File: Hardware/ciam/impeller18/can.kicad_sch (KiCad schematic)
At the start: 66 parts, among them J24 PLS-5, J25 PLS-5, J5 430450400, J6 430450400, SW4 MSS-12D16, SW5 MSS-12D16, U11 ISO1050DUB, U12 ISO1050DUB, U13 MCP2515-I/SO, U14 B0505MT-1WR4, U15 ISO1050DUB, U16 ISO1050DUB, U17 MCP2515-I/SO, U18 B0505MT-1WR4, Y3 X322516MLB4SI, Y4 X322516MLB4SI

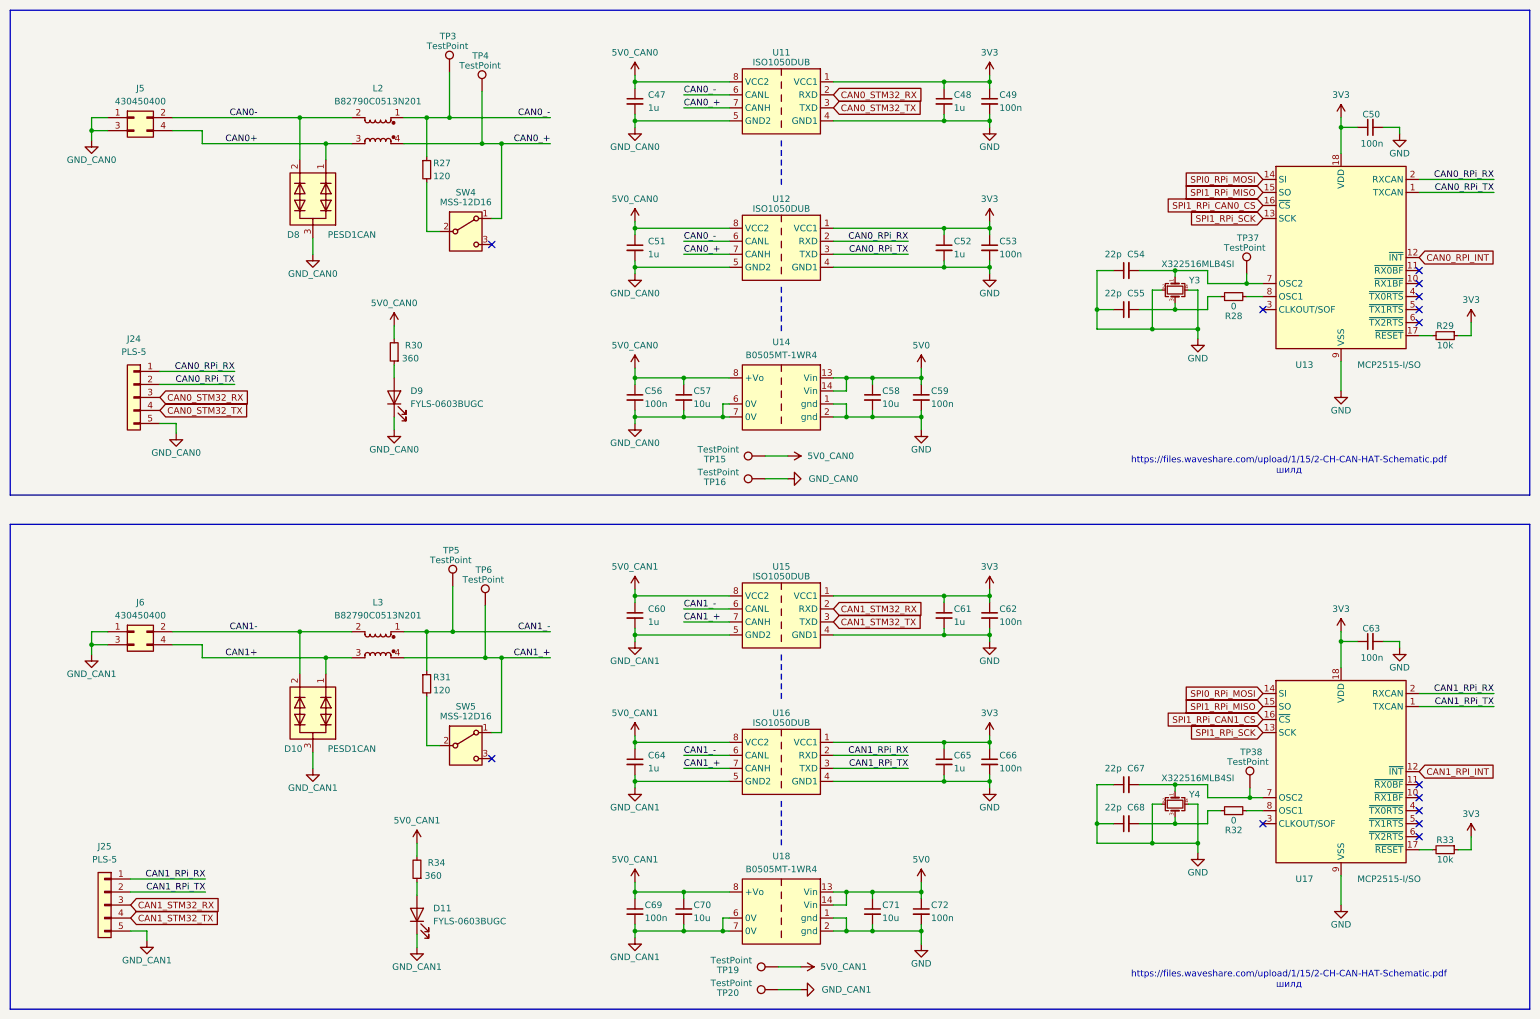
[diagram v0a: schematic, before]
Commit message: Minor changes
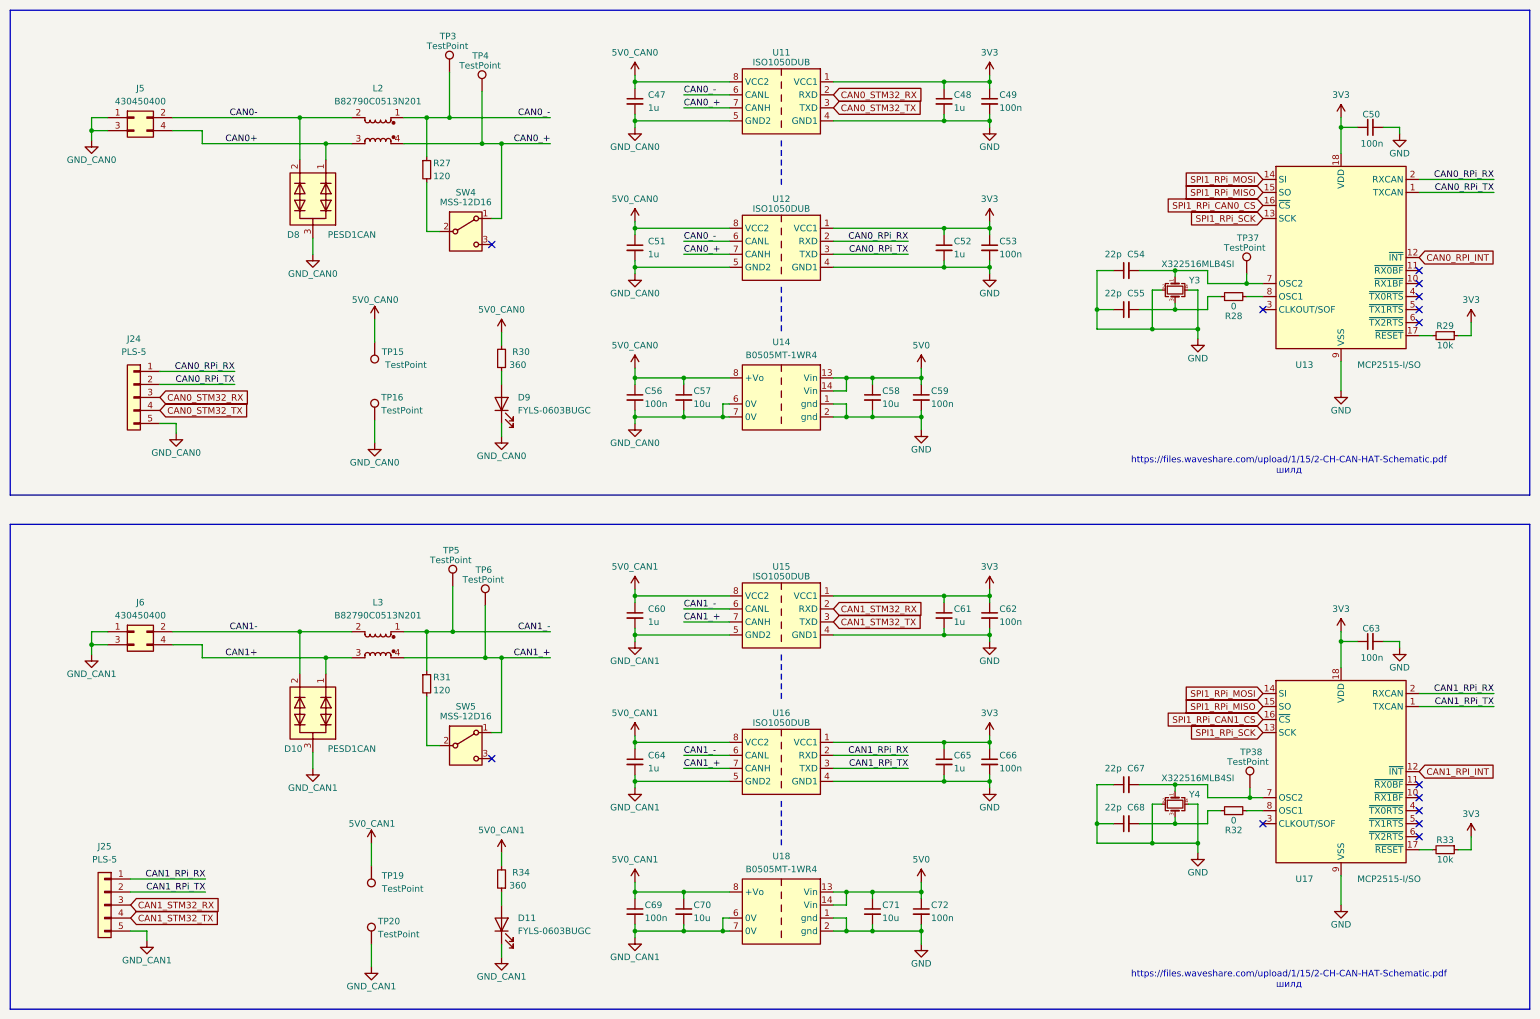
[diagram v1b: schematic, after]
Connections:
- net SPI0_RPi_MOSI renamed SPI1_RPi_MOSI
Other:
- moved on the sheet: D11, D9, R30, R34, TP15, TP16, TP19, TP20
